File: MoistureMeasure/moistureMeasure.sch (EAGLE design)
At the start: 8 parts, among them IC1 74HC14D, Q1 BC847BSMD

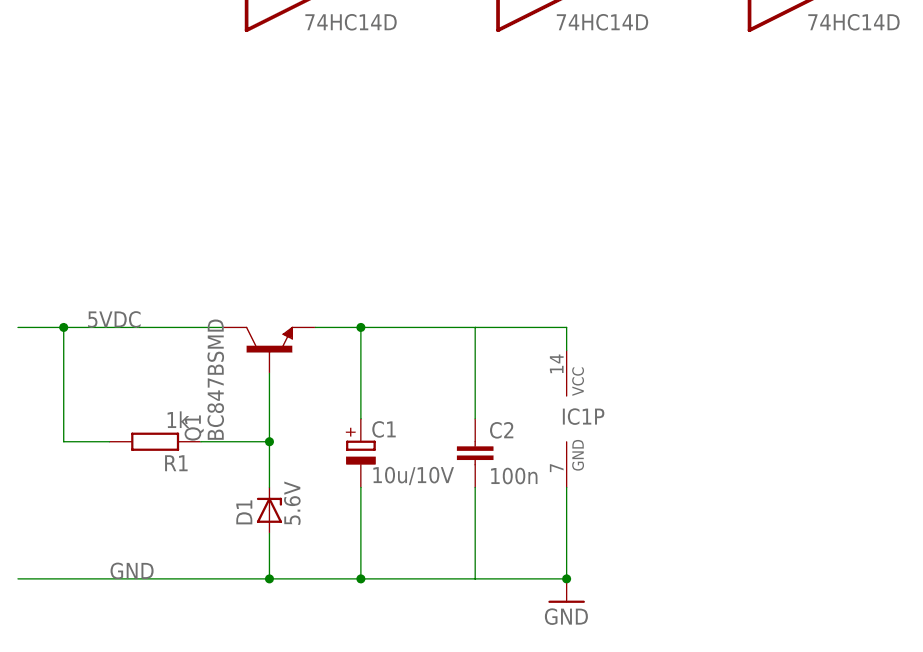
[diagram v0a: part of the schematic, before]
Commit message: some updates
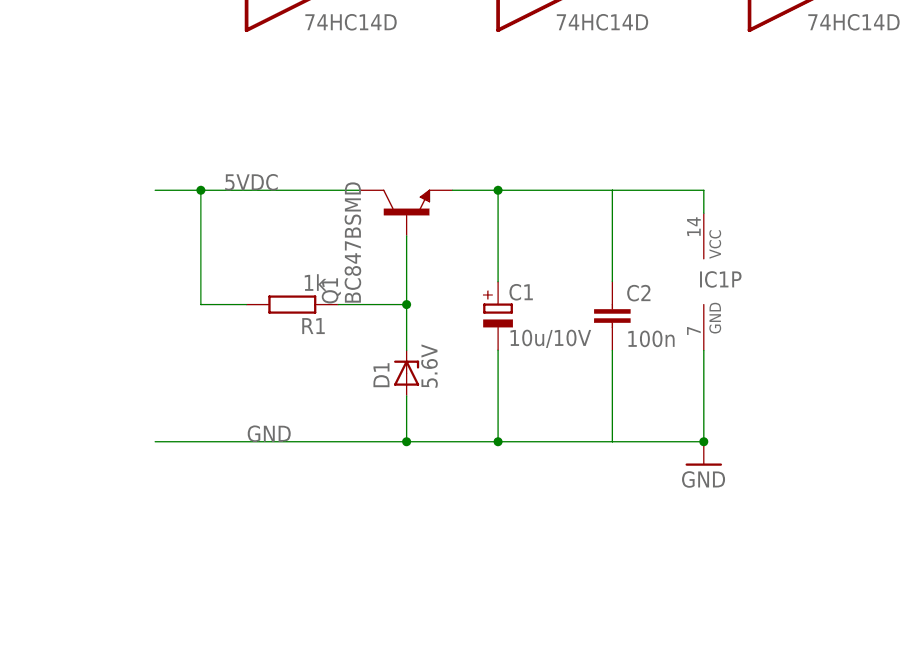
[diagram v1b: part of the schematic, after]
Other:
- moved on the sheet: C1, C2, D1, IC1P, Q1, R1
